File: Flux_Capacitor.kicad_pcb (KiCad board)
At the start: 2 copper layers, 35 x 30 mm, 23 parts, among them J1 ISP-6, SW1 SW_Push, U1 ATtiny13A-SU

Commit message: Set Design Rules
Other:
- net class Default: clearance 0.2 -> 0.1524; trace_width 0.25 -> 0.1524; via_dia 0.8 -> 0.508; via_drill 0.4 -> 0.254
- rule pad_to_mask_clearance: 0.051 -> 0.0508
- rule trace_clearance: 0.2 -> 0.1524
- rule trace_min: 0.2 -> 0.1524
- rule via_min_drill: 0.3 -> 0.254
- rule via_min_size: 0.4 -> 0.508
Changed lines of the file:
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@@
   )
   (page A4)
+  (title_block
+    (title "Flux Capacitor")
+    (date 2019-05-03)
+    (rev A)
+  )
   (layers
-    (0 F.Cu signal hide)
+    (0 F.Cu signal)
     (31 B.Cu signal)
     (32 B.Adhes user)
-    (33 F.Adhes user hide)
+    (33 F.Adhes user)
     (34 B.Paste user)
-    (35 F.Paste user hide)
+    (35 F.Paste user)
     (36 B.SilkS user)
-    (37 F.SilkS user hide)
+    (37 F.SilkS user)
     (38 B.Mask user)
-    (39 F.Mask user hide)
-    (40 Dwgs.User user hide)
-    (41 Cmts.User user hide)
-    (42 Eco1.User user hide)
-    (43 Eco2.User user hide)
+    (39 F.Mask user)
+    (40 Dwgs.User user)
+    (41 Cmts.User user)
+    (42 Eco1.User user)
+    (43 Eco2.User user)
     (44 Edge.Cuts user)
-    (45 Margin user hide)
-    (46 B.CrtYd user hide)
-    (47 F.CrtYd user hide)
-    (48 B.Fab user hide)
-    (49 F.Fab user hide)
+    (45 Margin user)
+    (46 B.CrtYd user)
+    (47 F.CrtYd user)
+    (48 B.Fab user)
+    (49 F.Fab user)
   )
   (setup
-    (last_trace_width 0.25)
-    (trace_clearance 0.2)
+    (last_trace_width 0.1524)
+    (trace_clearance 0.1524)
     (zone_clearance 0.508)
     (zone_45_only no)
-    (trace_min 0.2)
-    (via_size 0.8)
-    (via_drill 0.4)
-    (via_min_size 0.4)
-    (via_min_drill 0.3)
+    (trace_min 0.1524)
+    (via_size 0.508)
+    (via_drill 0.254)
+    (via_min_size 0.508)
+    (via_min_drill 0.254)
     (uvia_size 0.3)
     (uvia_drill 0.1)
@@
     (pad_size 1.524 1.524)
     (pad_drill 0.762)
-    (pad_to_mask_clearance 0.051)
+    (pad_to_mask_clearance 0.0508)
     (solder_mask_min_width 0.25)
     (aux_axis_origin 0 0)
-    (visible_elements FFFFF77F)
+    (visible_elements FFFFFF7F)
     (pcbplotparams
       (layerselection 0x010fc_ffffffff)
@@
   (net 20 "Net-(R2-Pad1)")
   (net_class Default "This is the default net class."
-    (clearance 0.2)
-    (trace_width 0.25)
-    (via_dia 0.8)
-    (via_drill 0.4)
+    (clearance 0.1524)
+    (trace_width 0.1524)
+    (via_dia 0.508)
+    (via_drill 0.254)
     (uvia_dia 0.3)
     (uvia_drill 0.1)

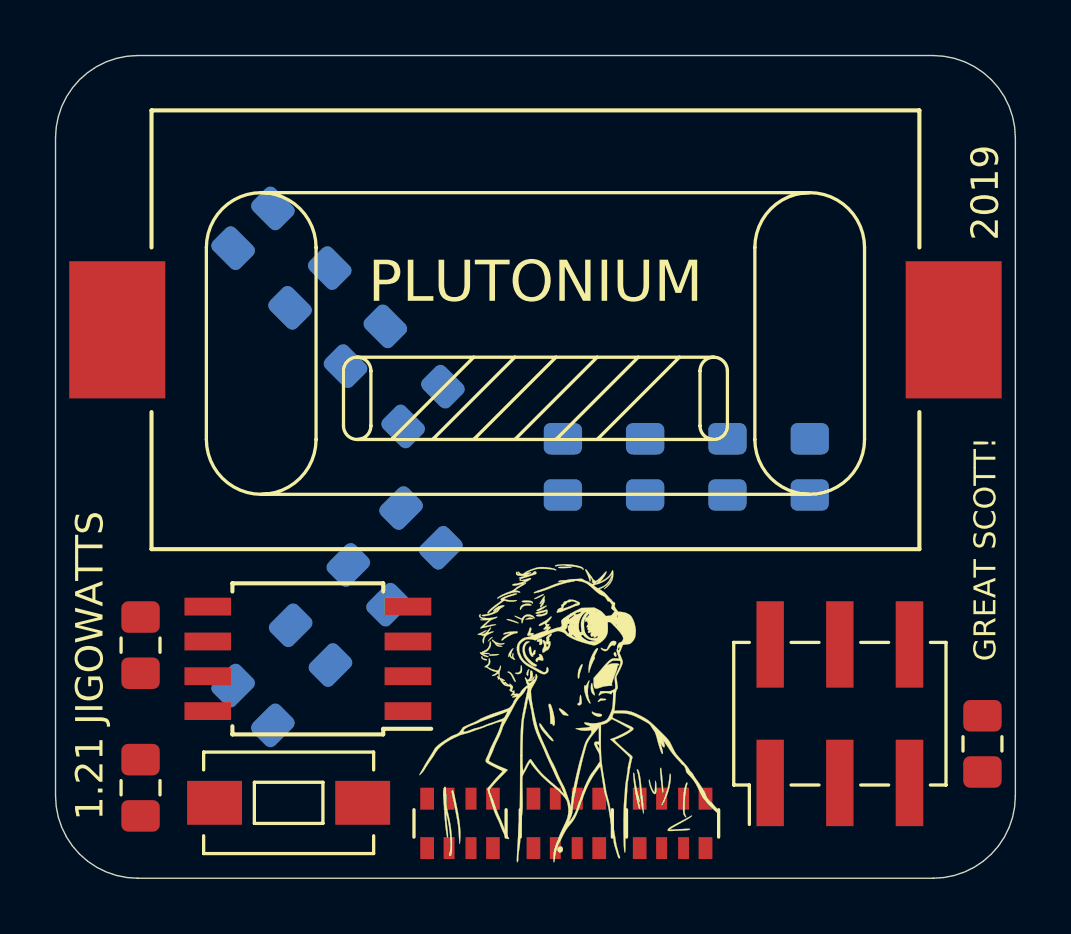
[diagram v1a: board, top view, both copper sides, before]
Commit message: Initial Routing
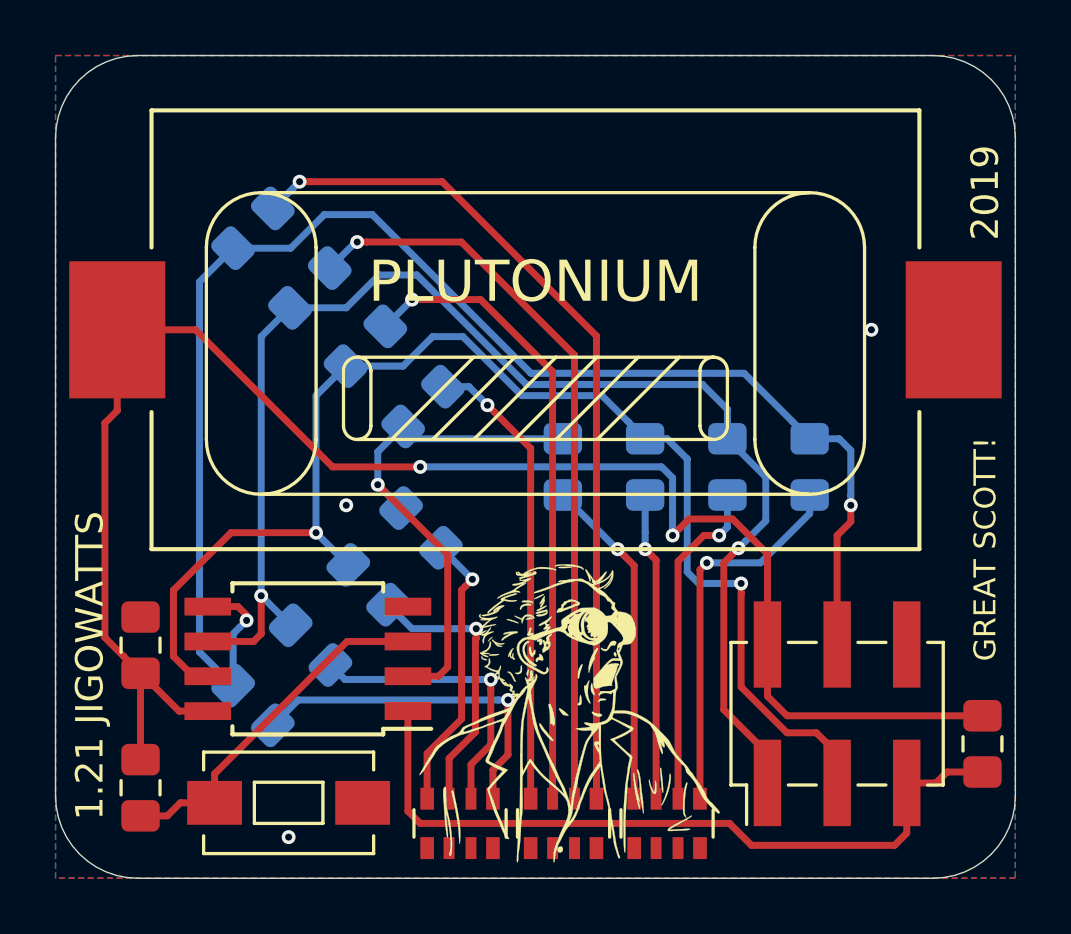
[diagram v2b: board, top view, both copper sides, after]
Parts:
- moved RN3 0.20 mm to (82.3, 78.0)
- moved J1 0.10 mm to (88.5, 74.0)
- moved RN2 0.10 mm to (78.5, 78.0)
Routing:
- net +3V0: track 0.00 -> 61.6 mm, vias 0 -> 2
- net /MOSI: track 0.00 -> 55.2 mm, vias 0 -> 2
- net /MISO: track 0.00 -> 49.9 mm, vias 0 -> 2
- net /SCK: track 0.00 -> 48.6 mm, vias 0 -> 2
- net Net-(D2-Pad1): track 0.00 -> 31.4 mm, vias 0 -> 1
- net /RST: track 0.00 -> 27.3 mm
- net Net-(D5-Pad1): track 0.00 -> 27.2 mm, vias 0 -> 1
- net Net-(D8-Pad1): track 0.00 -> 23.2 mm, vias 0 -> 1
- net Net-(D10-Pad2): track 0.00 -> 19.0 mm, vias 0 -> 1
- net Net-(D11-Pad1): track 0.00 -> 16.9 mm, vias 0 -> 1
- net Net-(D3-Pad1): track 0.00 -> 13.9 mm, vias 0 -> 1
- net Net-(R2-Pad1): track 0.00 -> 13.0 mm
- net Net-(D1-Pad1): track 0.00 -> 12.8 mm, vias 0 -> 1
- net Net-(D12-Pad1): track 0.00 -> 12.2 mm, vias 0 -> 1
- net Net-(D6-Pad1): track 0.00 -> 12.1 mm, vias 0 -> 1
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- added copper zone on B.Cu, net GND
- added copper zone on F.Cu, net GND
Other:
- net class Default: trace_width 0.1524 -> 0.254
